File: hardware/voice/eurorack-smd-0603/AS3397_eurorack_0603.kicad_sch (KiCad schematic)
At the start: 105 parts, among them J1 ES, Q1 BS170F, Q2 BS170F, Q3 BS170F, Q4 BS170F, Q5 BS170F, U1 MCP6002, U2 Pico, U3 MCP6002, U4 MCP6002, U5 MCP6002, U6 74HC4050, U7 MCP6002

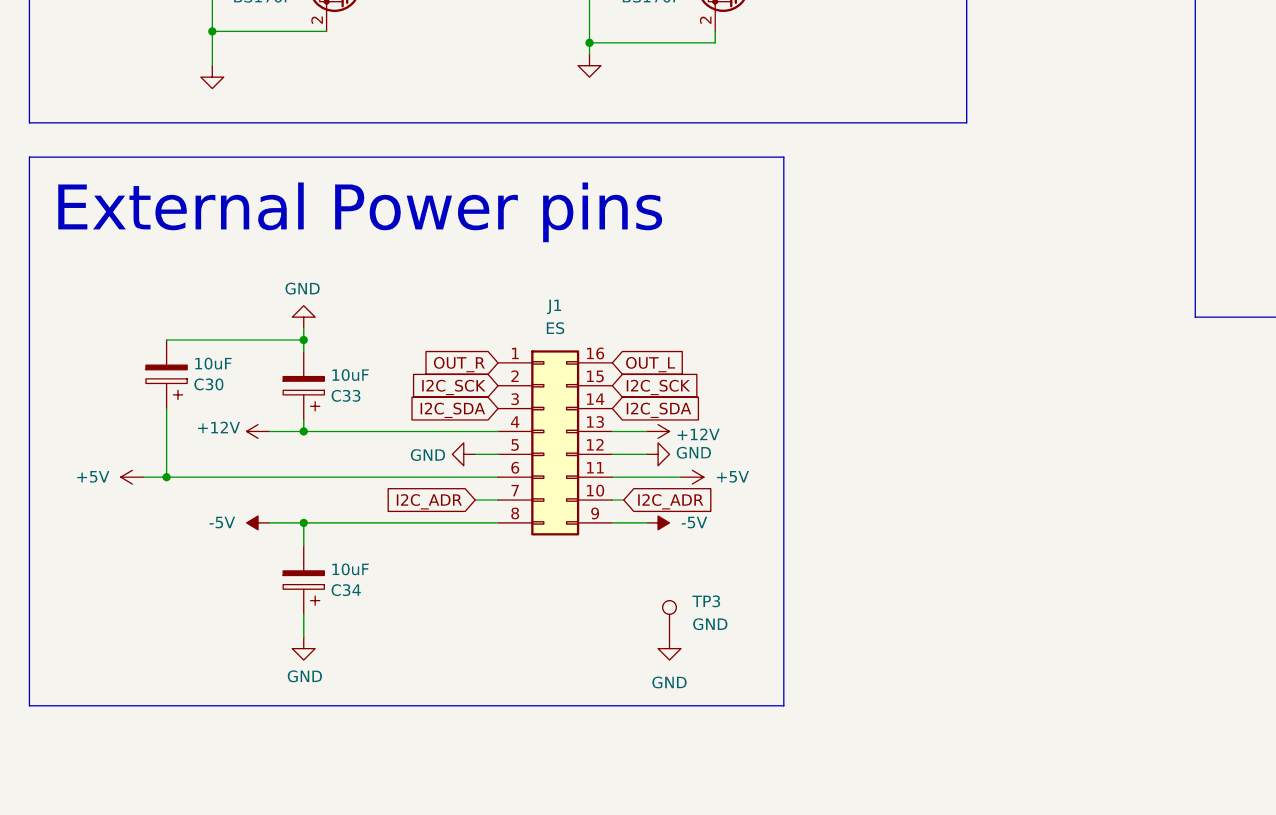
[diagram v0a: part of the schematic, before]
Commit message: Voice PCB directory cleanup
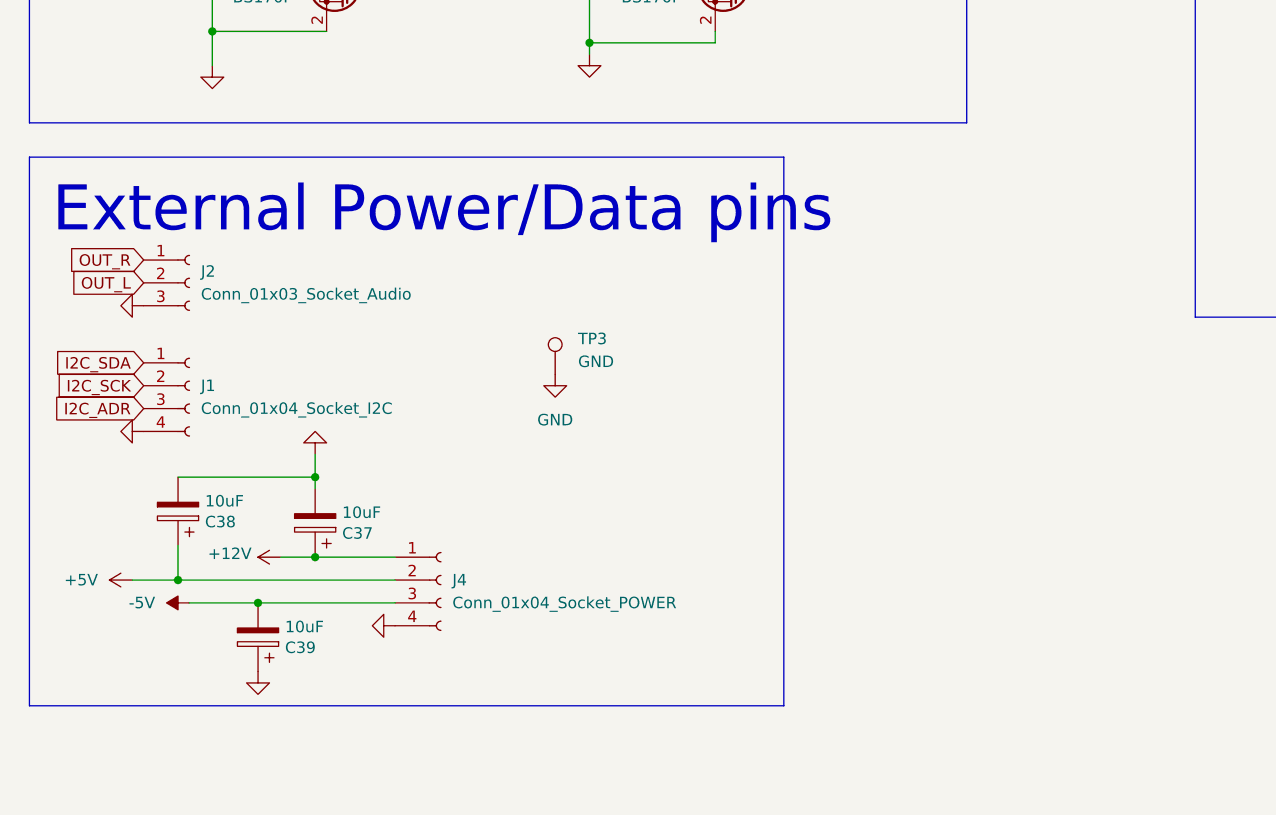
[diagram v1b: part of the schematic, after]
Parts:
- removed C30, C33, C34: 10uF, Capacitor_SMD:C_1206_3216Metric_Pad1.33x1.80mm_HandSolder, symbol VCF 3320-rescue:CP-Device
- removed J1: ES, SYNTHFILLE:DIP-16_AS, symbol Connector_Generic:Conn_02x08_Counter_Clockwise
- added C37, C38, C39: 10uF, Capacitor_SMD:C_0603_1608Metric_Pad1.08x0.95mm_HandSolder, symbol VCF 3320-rescue:CP-Device
- added J1: Conn_01x04_Socket_I2C, Connector_PinHeader_2.54mm:PinHeader_1x04_P2.54mm_Vertical, symbol Connector:Conn_01x04_Socket
- added J2: Conn_01x03_Socket_Audio, Connector_PinHeader_2.54mm:PinHeader_1x03_P2.54mm_Vertical, symbol Connector:Conn_01x03_Socket
- added J4: Conn_01x04_Socket_POWER, Connector_PinHeader_2.54mm:PinHeader_1x04_P2.54mm_Vertical, symbol Connector:Conn_01x04_Socket
- C1, C11, C12, C15, C16, C17, C18, C19, C2, C20, C21, C22, C23, C24, C25, C26, C27, C28, C29, C3, C31, C32, C35, C36, C4, C5, C6, C7, C8, C9: footprint Capacitor_SMD:C_1206_3216Metric_Pad1.33x1.80mm_HandSolder -> Capacitor_SMD:C_0603_1608Metric_Pad1.08x0.95mm_HandSolder
- C10, C13, C14: footprint Capacitor_SMD:C_0805_2012Metric_Pad1.18x1.45mm_HandSolder -> Capacitor_SMD:C_0603_1608Metric_Pad1.08x0.95mm_HandSolder
- R1, R10, R11, R12, R13, R14, R15, R16, R17, R18, R19, R2, R20, R21, R22, R23, R24, R25, R26, R27, R28, R29, R3, R30, R31, R32, R33, R34, R35, R36, R37, R38, R39, R4, R40, R41, R42, R43, R44, R45, R46, R47, R48, R49, R5, R6, R7, R8, R9: footprint Resistor_SMD:R_1206_3216Metric_Pad1.30x1.75mm_HandSolder -> Resistor_SMD:R_0603_1608Metric_Pad0.98x0.95mm_HandSolder
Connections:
- net +12V: now also C37.1, J4.1 (Pin_1)
- net +5V: now also C38.1, J4.2 (Pin_2)
- net -5V: now also C39.2, J4.3 (Pin_3)
- net GND: now also C37.2, C38.2, C39.1, J1.4 (Pin_4), J2.3 (Pin_3), J4.4 (Pin_4)
- net I2C_ADR: now also J1.3 (Pin_3)
- net I2C_SCK: now also J1.2 (Pin_2)
- net I2C_SDA: now also J1.1 (Pin_1)
- net OUT_L: now also J2.2 (Pin_2)
- net OUT_R: now also J2.1 (Pin_1)
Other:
- note added: "External Power/Data pins"
- note removed: "External Power pins"
- moved on the sheet: TP3

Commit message: Voice PCB directory cleanup bis
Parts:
- C3, C37, C38, C39: footprint Capacitor_SMD:C_0603_1608Metric_Pad1.08x0.95mm_HandSolder -> Capacitor_SMD:C_1206_3216Metric_Pad1.33x1.80mm_HandSolder
- U2: footprint SYNTHFILLE:RPi_Pico_SMD_AS -> AS3397_eurorack_0603:RPi_Pico_SMD_TH
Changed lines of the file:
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@@
       (effects (font (size 1.27 1.27)) (justify right))
     )
-    (property "Footprint" "Capacitor_SMD:C_0603_1608Metric_Pad1.08x0.95mm_HandSolder" (at 46.0248 373.38 0)
+    (property "Footprint" "Capacitor_SMD:C_1206_3216Metric_Pad1.33x1.80mm_HandSolder" (at 46.0248 373.38 0)
       (effects (font (size 1.27 1.27)) hide)
     )
@@
       (effects (font (size 1.27 1.27)) (justify right))
     )
-    (property "Footprint" "Capacitor_SMD:C_0603_1608Metric_Pad1.08x0.95mm_HandSolder" (at 39.6748 386.08 0)
+    (property "Footprint" "Capacitor_SMD:C_1206_3216Metric_Pad1.33x1.80mm_HandSolder" (at 39.6748 386.08 0)
       (effects (font (size 1.27 1.27)) hide)
     )
@@
       (effects (font (size 1.27 1.27)) (justify right))
     )
-    (property "Footprint" "Capacitor_SMD:C_0603_1608Metric_Pad1.08x0.95mm_HandSolder" (at 30.7848 372.11 0)
+    (property "Footprint" "Capacitor_SMD:C_1206_3216Metric_Pad1.33x1.80mm_HandSolder" (at 30.7848 372.11 0)
       (effects (font (size 1.27 1.27)) hide)
     )
@@
       (effects (font (size 1.27 1.27)))
     )
-    (property "Footprint" "Capacitor_SMD:C_0603_1608Metric_Pad1.08x0.95mm_HandSolder" (at 124.46 51.1048 0)
+    (property "Footprint" "Capacitor_SMD:C_1206_3216Metric_Pad1.33x1.80mm_HandSolder" (at 124.46 51.1048 0)
       (effects (font (size 1.27 1.27)) hide)
     )
@@
       (effects (font (size 1.27 1.27)))
     )
-    (property "Footprint" "SYNTHFILLE:RPi_Pico_SMD_AS" (at 74.93 158.75 90)
+    (property "Footprint" "AS3397_eurorack_0603:RPi_Pico_SMD_TH" (at 74.93 158.75 90)
       (effects (font (size 1.27 1.27)) hide)
     )
